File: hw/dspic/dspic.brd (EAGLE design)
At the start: 61.9 x 40.6 mm, 25 parts, among them Q1 8MHz, U1 DSPIC33FJ128MC802-I/SP

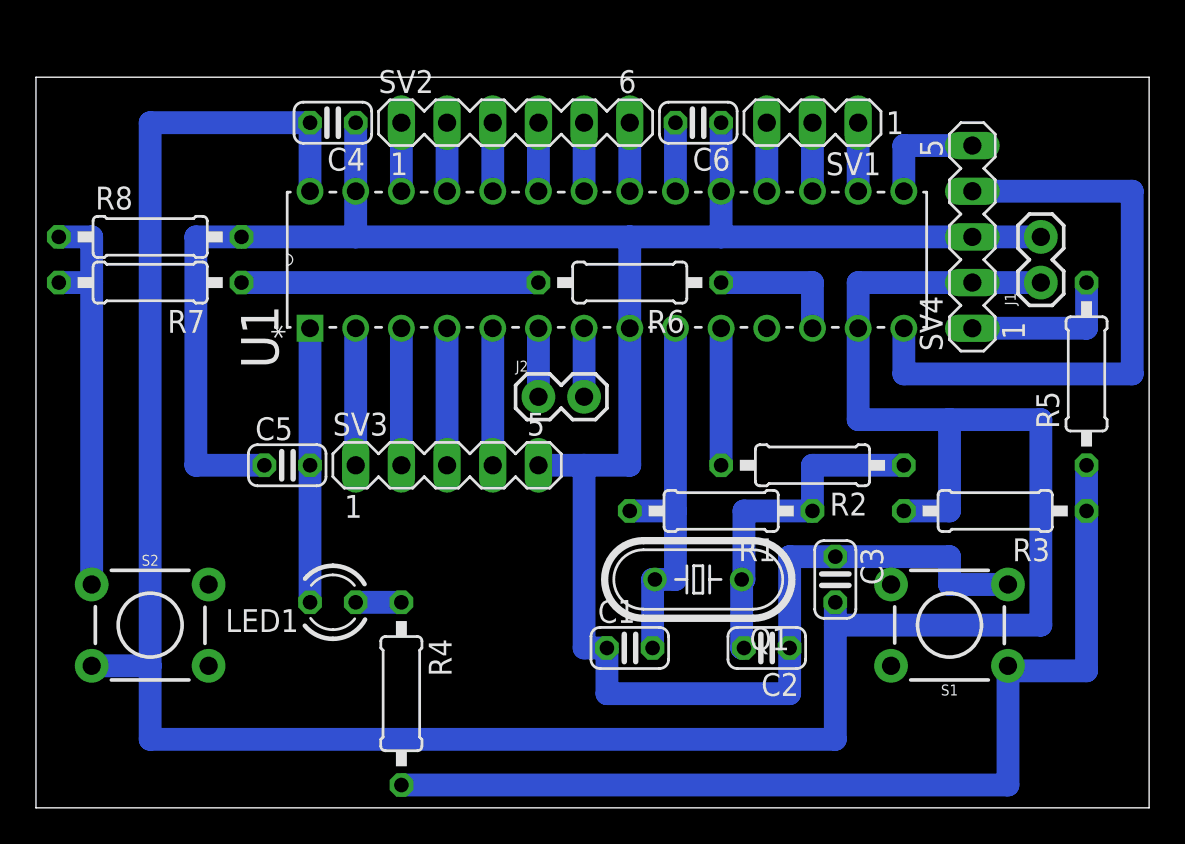
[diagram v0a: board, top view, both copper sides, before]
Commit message: layout
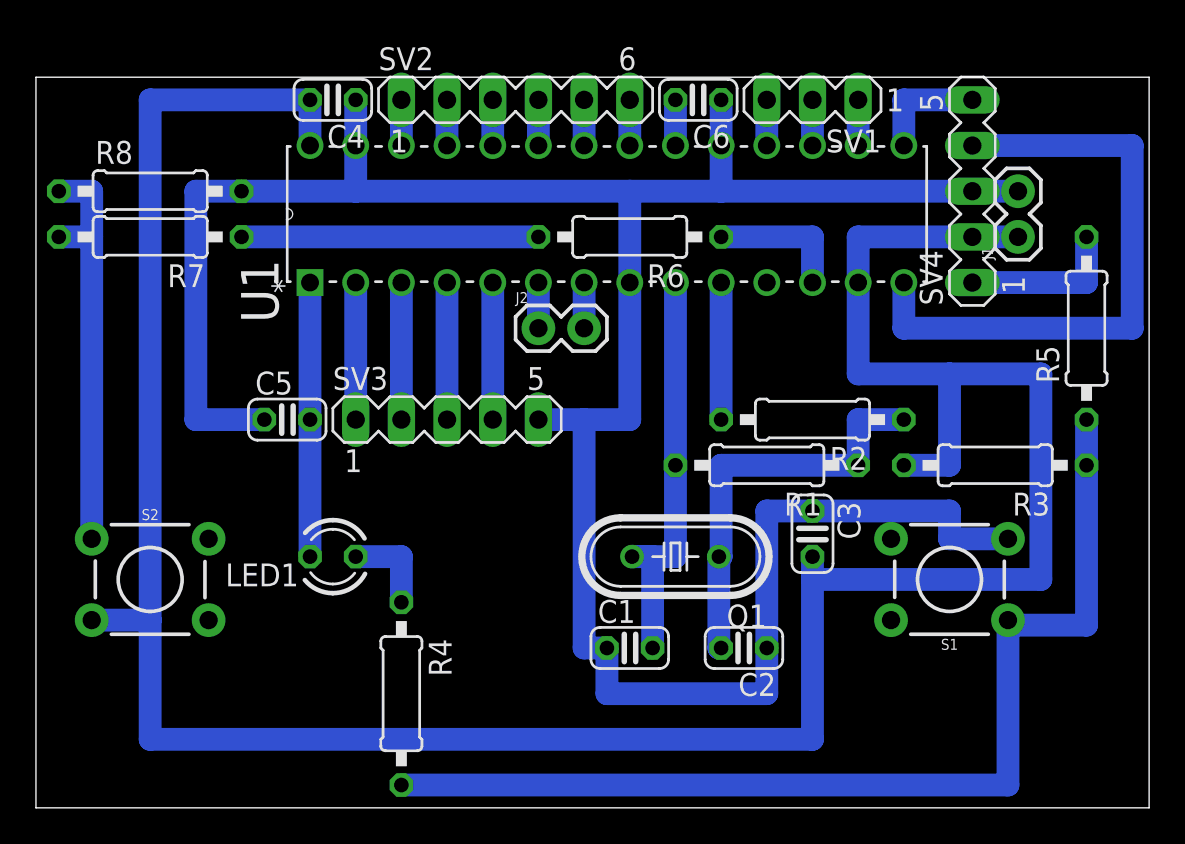
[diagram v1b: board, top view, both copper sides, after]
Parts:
- moved J2 3.81 mm to (27.9, 26.7)
- moved R1 3.59 mm to (40.6, 19.1)
- moved C3 2.84 mm to (43.2, 15.2)
- moved J1 2.84 mm to (54.6, 31.8)
- moved R5 2.54 mm to (58.4, 26.7)
- moved U1 2.54 mm to (31.8, 33.0)
- moved LED1 2.54 mm to (16.5, 14.0)
- moved C5 2.54 mm to (14.0, 21.6)
- moved R2 2.54 mm to (43.2, 21.6)
- moved R3 2.54 mm to (53.3, 19.1)
- moved R6 2.54 mm to (33.0, 31.8)
- moved R7 2.54 mm to (6.35, 31.8)
- moved R8 2.54 mm to (6.35, 34.3)
- moved S1 2.54 mm to (50.8, 12.7)
- moved S2 2.54 mm to (6.35, 12.7)
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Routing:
- net N$8: track 19.3 -> 23.1 mm
- net N$5: track 2.54 -> 5.08 mm
- net N$4: track 56.2 -> 58.7 mm
- net N$7: track 21.6 -> 23.9 mm
- net GND: track 139.4 -> 140.7 mm
- net +3V3: track 154.4 -> 155.7 mm
- net U1TX: track 3.81 -> 2.54 mm
- net U1RX: track 3.81 -> 2.54 mm
- net N$11: track 3.81 -> 2.54 mm
- net N$10: track 3.81 -> 2.54 mm
- net N$1: track 3.81 -> 2.54 mm
- net L3: track 3.81 -> 2.54 mm
- net L2: track 3.81 -> 2.54 mm
- net L1: track 3.81 -> 2.54 mm
- net INT0: track 3.81 -> 2.54 mm
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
